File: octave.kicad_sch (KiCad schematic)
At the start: 25 parts, among them Q3 2N3904, Q4 2N3904, Q5 2N3904

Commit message: Adctualización de PCB
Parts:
- D1, D2: footprint Diode_THT:D_DO-35_SOD27_P7.62mm_Horizontal -> DIY_jorge:D_DO-35_SOD27_P7.62mm_Horizontal
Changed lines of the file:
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@@
 			)
 		)
-		(property "Footprint" "Diode_THT:D_DO-35_SOD27_P7.62mm_Horizontal"
+		(property "Footprint" "DIY_jorge:D_DO-35_SOD27_P7.62mm_Horizontal"
 			(at 220.98 88.9 0)
 			(effects
@@
 			)
 		)
-		(property "Footprint" "Diode_THT:D_DO-35_SOD27_P7.62mm_Horizontal"
+		(property "Footprint" "DIY_jorge:D_DO-35_SOD27_P7.62mm_Horizontal"
 			(at 208.28 88.9 0)
 			(effects

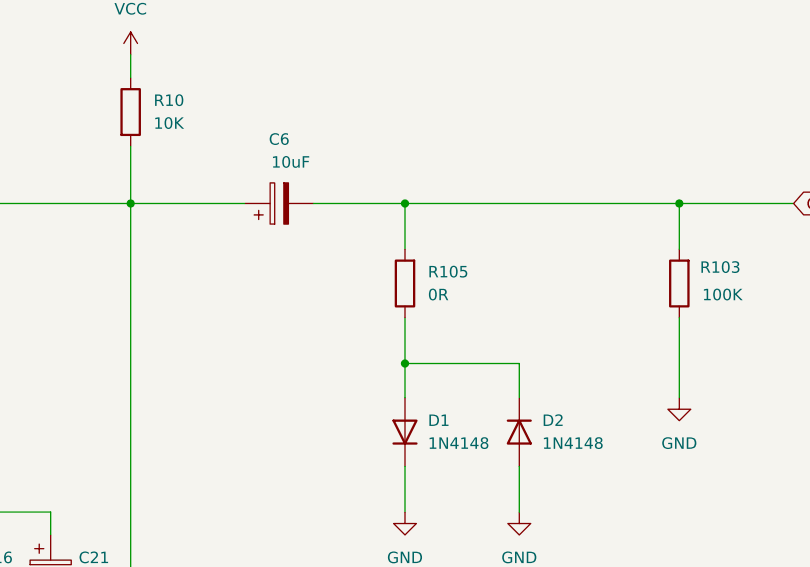
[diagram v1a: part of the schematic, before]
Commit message: Finalización de PCB (archivos fabricación pendientes)
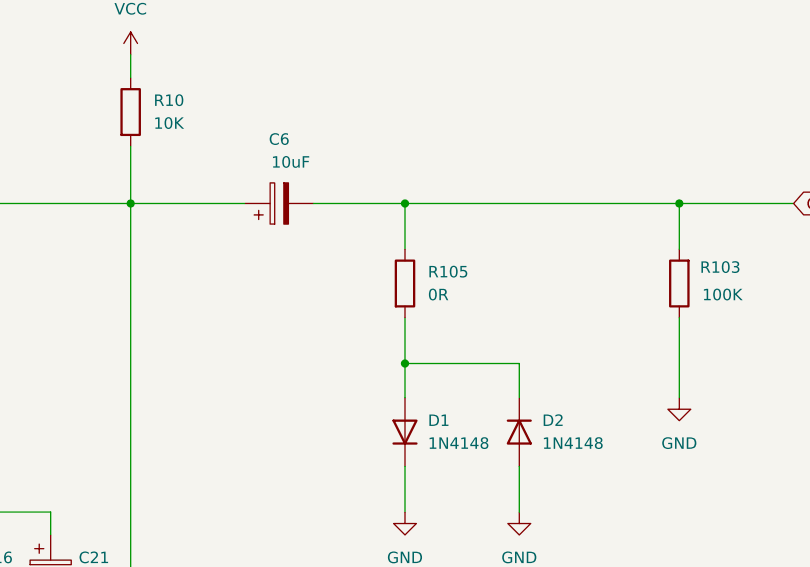
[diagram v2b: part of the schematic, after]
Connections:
- net OCTAVE_OUT: now also R105.1; no longer R105.2
- net at D1.2 (A), D2.1 (K): now also R105.2; no longer R105.1
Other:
- moved on the sheet: R105
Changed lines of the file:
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@@
 	(symbol
 		(lib_id "Device:R")
-		(at 208.28 72.39 180)
+		(at 208.28 72.39 0)
 		(unit 1)
 		(exclude_from_sim no)
@@
 					(size 1.27 1.27)
 				)
-				(justify right)
+				(justify left)
 			)
 		)
@@
 					(size 1.27 1.27)
 				)
-				(justify right)
+				(justify left)
 			)
 		)
 		(property "Footprint" "Resistor_THT:R_Axial_DIN0207_L6.3mm_D2.5mm_P7.62mm_Horizontal"
-			(at 210.058 72.39 90)
+			(at 206.502 72.39 90)
 			(effects
 				(font
